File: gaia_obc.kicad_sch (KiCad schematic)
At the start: 57 parts, among them J1 USB_C_Receptacle_USB2.0_16P, J2 Conn_02x10_Odd_Even, J3 Conn_02x10_Odd_Even, Q1 IRLML6244, SW1 SW_Push, SW2 SW_Push, U1 MCP23017_ML, U2 USBLC6-2P6, U3 ESP32-S3-PICO-1-N8R2

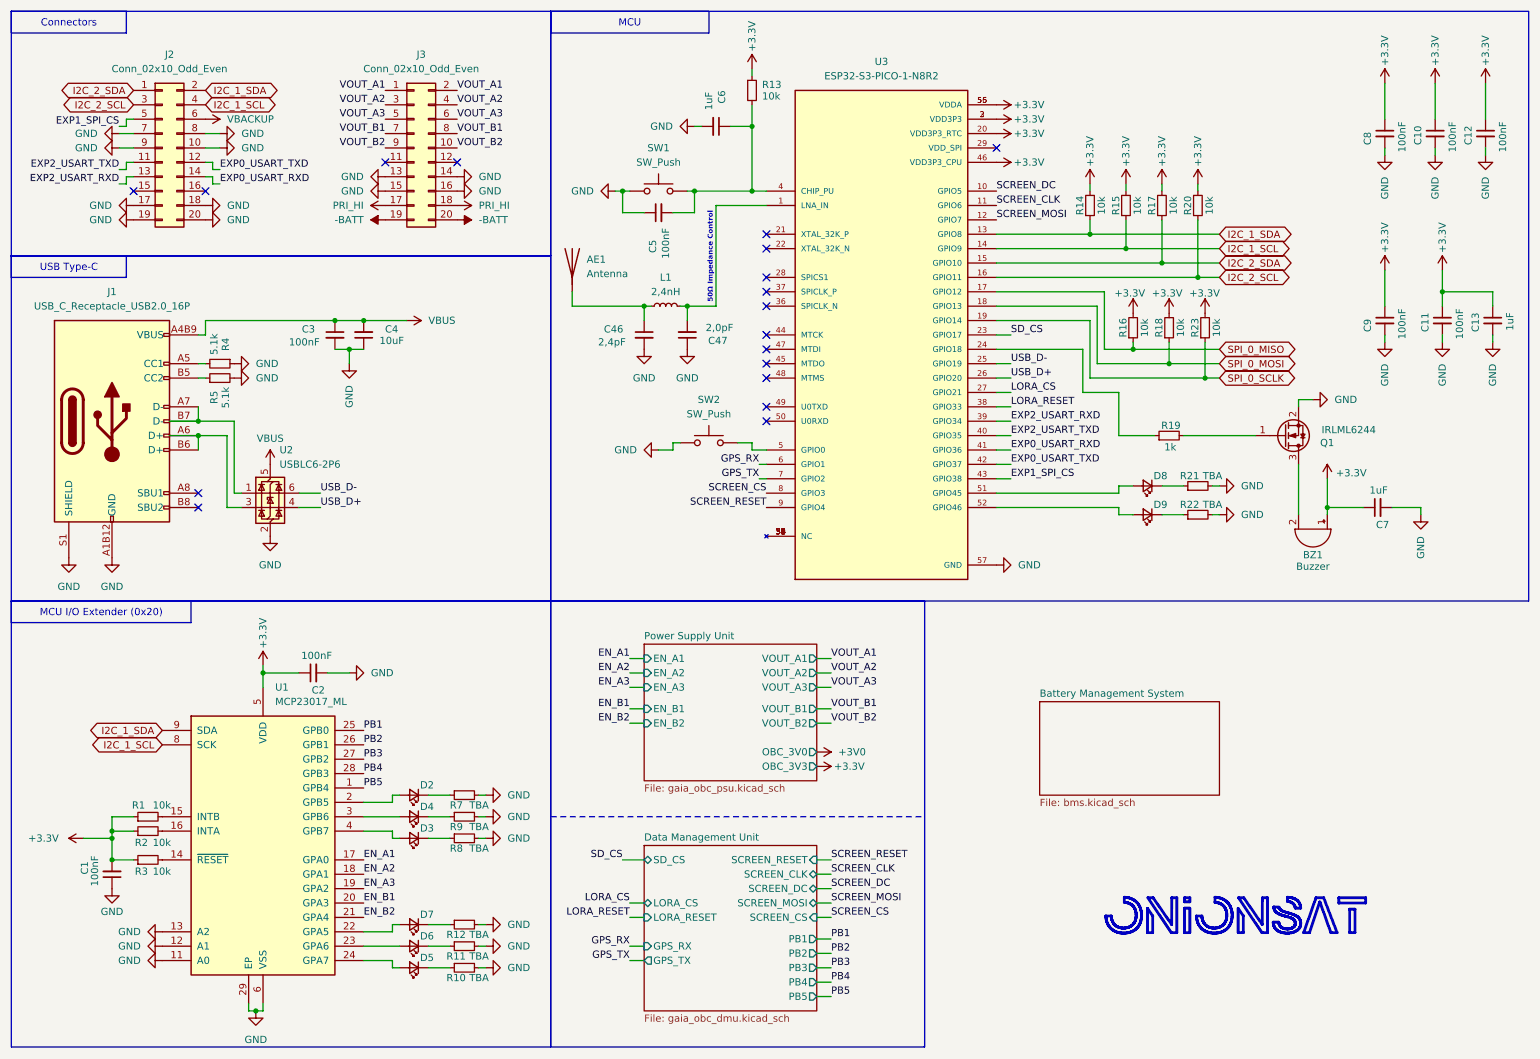
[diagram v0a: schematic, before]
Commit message: neptune 1.3 production
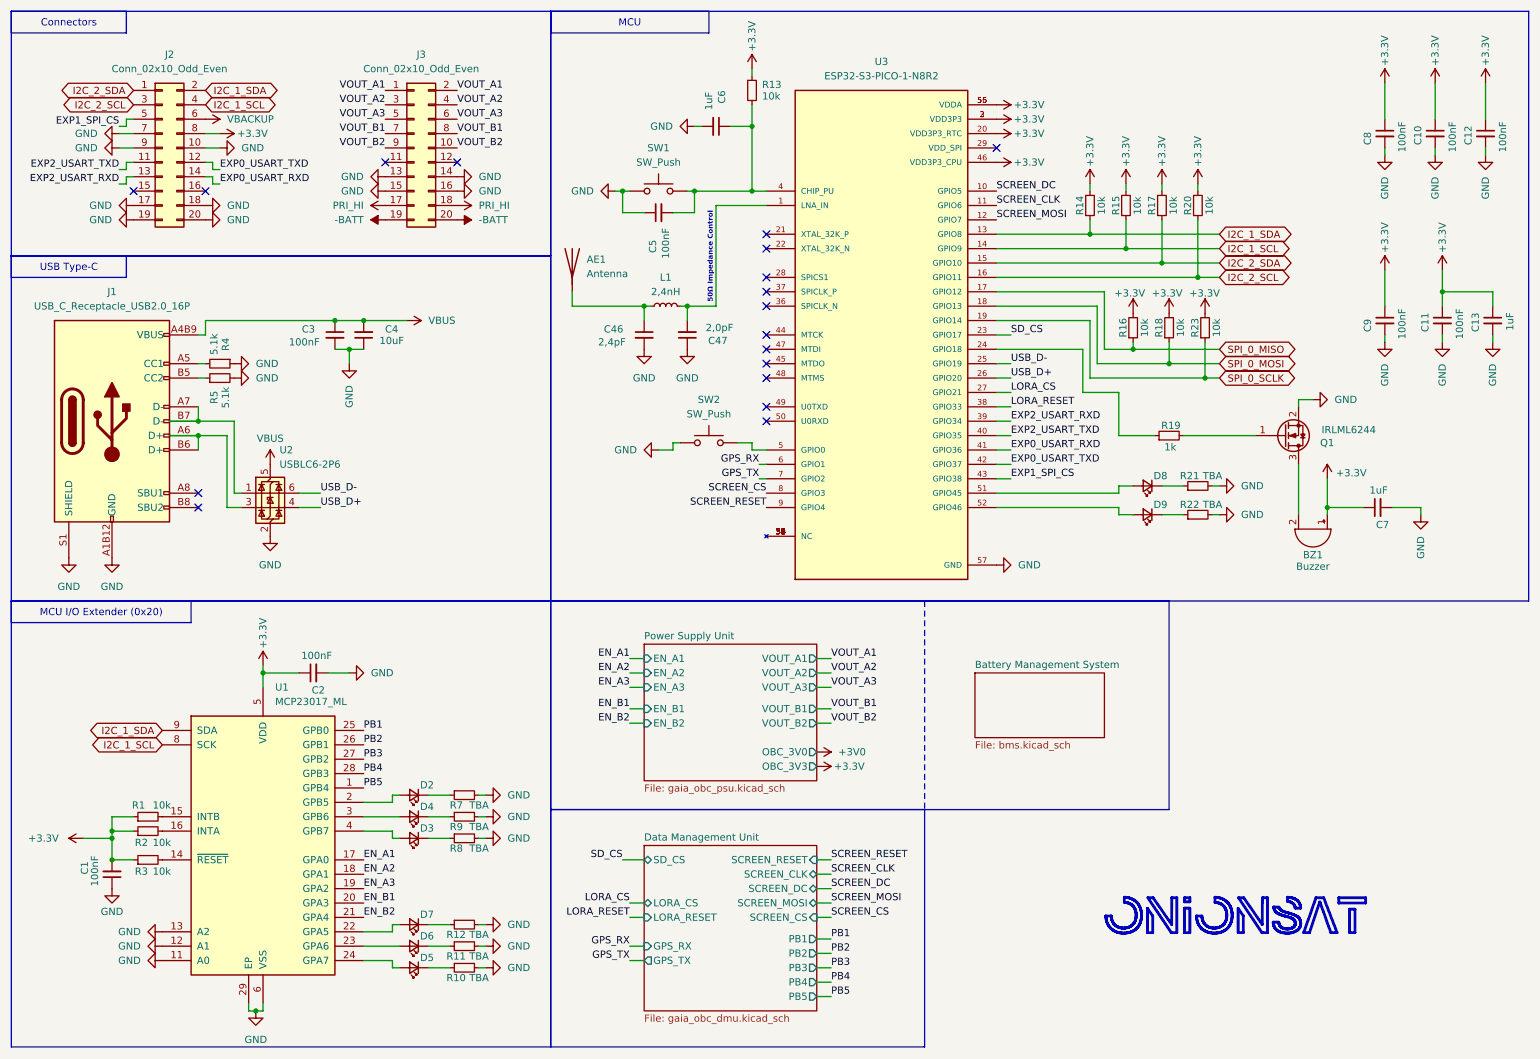
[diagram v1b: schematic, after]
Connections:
- net +3.3V: now also J2.8 (Pin_8)
- net GND: no longer J2.8 (Pin_8)
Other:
- title: GAIA On-Board Computer -> Neptune On-Board Computer
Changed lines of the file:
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@@
 	(paper "A4")
 	(title_block
-		(title "GAIA On-Board Computer")
-		(date "2025-12-01")
-		(rev "1.2")
+		(title "Neptune On-Board Computer")
+		(date "2025-12-12")
+		(rev "1.3")
 	)
 	(polyline
@@
 			(width 0.5)
 			(type solid)
+			(color 0 0 0 1)
 		)
 		(fill
 			(type color)
-			(color 0 0 0 0)
+			(color 0 0 0 1)
 		)
 	)
@@
 			(width 0.5)
 			(type solid)
+			(color 0 0 0 1)
 		)
 		(fill
 			(type color)
-			(color 0 0 0 0)
+			(color 0 0 0 1)
 		)
 	)
@@
 			(width 0.5)
 			(type solid)
+			(color 0 0 0 1)
 		)
 		(fill
 			(type color)
-			(color 0 0 0 0)
+			(color 0 0 0 1)
 		)
 	)
@@
 			(width 0.5)
 			(type solid)
+			(color 0 0 0 1)
 		)
 		(fill
 			(type color)
-			(color 0 0 0 0)
+			(color 0 0 0 1)
+		)
+	)
+	(rectangle
+		(start 109.22 154.94)
+		(end 175.26 196.85)
+		(stroke
+			(width 0)
+			(type default)
+		)
+		(fill
+			(type none)
 		)
 	)
@@
 			(width 0.5)
 			(type solid)
+			(color 0 0 0 1)
 		)
 		(fill
 			(type color)
-			(color 0 0 0 0)
+			(color 0 0 0 1)
 		)
 	)
@@
 			(width 0.5)
 			(type solid)
+			(color 0 0 0 1)
 		)
 		(fill
 			(type color)
-			(color 0 0 0 0)
+			(color 0 0 0 1)
 		)
 	)
@@
 			(width 0.5)
 			(type solid)
+			(color 0 0 0 1)
 		)
 		(fill
 			(type color)
-			(color 0 0 0 0)
+			(color 0 0 0 1)
 		)
 	)
 	(rectangle
 		(start 109.22 118.11)
-		(end 175.26 196.85)
+		(end 218.44 154.94)
 		(stroke
 			(width 0)
@@
 			(width 0.5)
 			(type solid)
+			(color 0 0 0 1)
 		)
 		(fill
 			(type color)
-			(color 0 0 0 0)
+			(color 0 0 0 1)
 		)
 	)
@@
 			(width 0.5)
 			(type solid)
+			(color 0 0 0 1)
 		)
 		(fill
 			(type color)
-			(color 0 0 0 0)
+			(color 0 0 0 1)
 		)
 	)
@@
 			(width 0.5)
 			(type solid)
+			(color 0 0 0 1)
 		)
 		(fill
 			(type color)
-			(color 0 0 0 0)
+			(color 0 0 0 1)
 		)
 	)
@@
 			(width 0.5)
 			(type solid)
+			(color 0 0 0 1)
 		)
 		(fill
 			(type color)
-			(color 0 0 0 0)
+			(color 0 0 0 1)
 		)
 	)
@@
 			(width 0.5)
 			(type solid)
+			(color 0 0 0 1)
 		)
 		(fill
 			(type color)
-			(color 0 0 0 0)
+			(color 0 0 0 1)
 		)
 	)
@@
 			(width 0.5)
 			(type solid)
+			(color 0 0 0 1)
 		)
 		(fill
 			(type color)
-			(color 0 0 0 0)
+			(color 0 0 0 1)
 		)
 	)
@@
 	(polyline
 		(pts
-			(xy 109.22 156.21) (xy 175.26 156.21)
+			(xy 175.26 118.11) (xy 175.26 154.94)
 		)
 		(stroke
@@
 	(symbol
 		(lib_id "power:GND")
-		(at 50.8 35.56 90)
-		(unit 1)
-		(exclude_from_sim no)
-		(in_bom yes)
-		(on_board yes)
-		(dnp no)
-		(fields_autoplaced yes)
-		(property "Reference" "#PWR0113"
-			(at 57.15 35.56 0)
-			(effects
-				(font
-					(size 1.27 1.27)
-				)
-				(hide yes)
-			)
-		)
-		(property "Value" "GND"
-			(at 54.61 35.5599 90)
-			(effects
-				(font
-					(size 1.27 1.27)
-				)
-				(justify right)
-			)
-		)
-		(property "Footprint" ""
-			(at 50.8 35.56 0)
-			(effects
-				(font
-					(size 1.27 1.27)
-				)
-				(hide yes)
-			)
-		)
-		(property "Datasheet" ""
-			(at 50.8 35.56 0)
-			(effects
-				(font
-					(size 1.27 1.27)
-				)
-				(hide yes)
-			)
-		)
-		(property "Description" "Power symbol creates a global label with name \"GND\" , ground"
-			(at 50.8 35.56 0)
-			(effects
-				(font
-					(size 1.27 1.27)
-				)
-				(hide yes)
-			)
-		)
-		(pin "1"
-		)
-		(instances
-			(project "gaia_obc"
-				(path "/049f7784-e0f9-4d41-b308-330ac61e4408"
-					(reference "#PWR0113")
-					(unit 1)
-				)
-			)
-		)
-	)
-	(symbol
-		(lib_id "power:GND")
 		(at 274.32 39.37 0)
 		(unit 1)
@@
 	)
 	(symbol
+		(lib_id "power:+3.3V")
+		(at 50.8 35.56 270)
+		(unit 1)
+		(exclude_from_sim no)
+		(in_bom yes)
+		(on_board yes)
+		(dnp no)
+		(property "Reference" "#PWR0113"
+			(at 46.99 35.56 0)
+			(effects
+				(font
+					(size 1.27 1.27)
+				)
+				(hide yes)
+			)
+		)
+		(property "Value" "+3.3V"
+			(at 53.848 35.56 90)
+			(effects
+				(font
+					(size 1.27 1.27)
+				)
+				(justify left)
+			)
+		)
+		(property "Footprint" ""
+			(at 50.8 35.56 0)
+			(effects
+				(font
+					(size 1.27 1.27)
+				)
+				(hide yes)
+			)
+		)
+		(property "Datasheet" ""
+			(at 50.8 35.56 0)
+			(effects
+				(font
+					(size 1.27 1.27)
+				)
+				(hide yes)
+			)
+		)
+		(property "Description" "Power symbol creates a global label with name \"+3.3V\""
+			(at 50.8 35.56 0)
+			(effects
+				(font
+					(size 1.27 1.27)
+				)
+				(hide yes)
+			)
+		)
+		(pin "1"
+		)
+		(instances
+			(project "gaia_obc"
+				(path "/049f7784-e0f9-4d41-b308-330ac61e4408"
+					(reference "#PWR0113")
+					(unit 1)
+				)
+			)
+		)
+	)
+	(symbol
 		(lib_id "power:GND")
 		(at 120.65 45.72 270)
@@
 	)
 	(sheet
-		(at 195.58 135.89)
-		(size 31.75 16.51)
+		(at 184.15 130.81)
+		(size 22.86 11.43)
 		(exclude_from_sim no)
 		(in_bom yes)
@@
 		)
 		(property "Sheetname" "Battery Management System"
-			(at 195.58 135.1784 0)
+			(at 184.15 130.0984 0)
 			(effects
 				(font
@@
 		)
 		(property "Sheetfile" "bms.kicad_sch"
-			(at 195.58 152.9846 0)
+			(at 184.15 142.8246 0)
 			(effects
 				(font
